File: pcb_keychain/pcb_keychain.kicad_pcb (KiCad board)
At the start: 11 copper layers, 84.3 x 60.5 mm, 7 parts, among them Q1 PN2222A, SW1 SW_SPDT

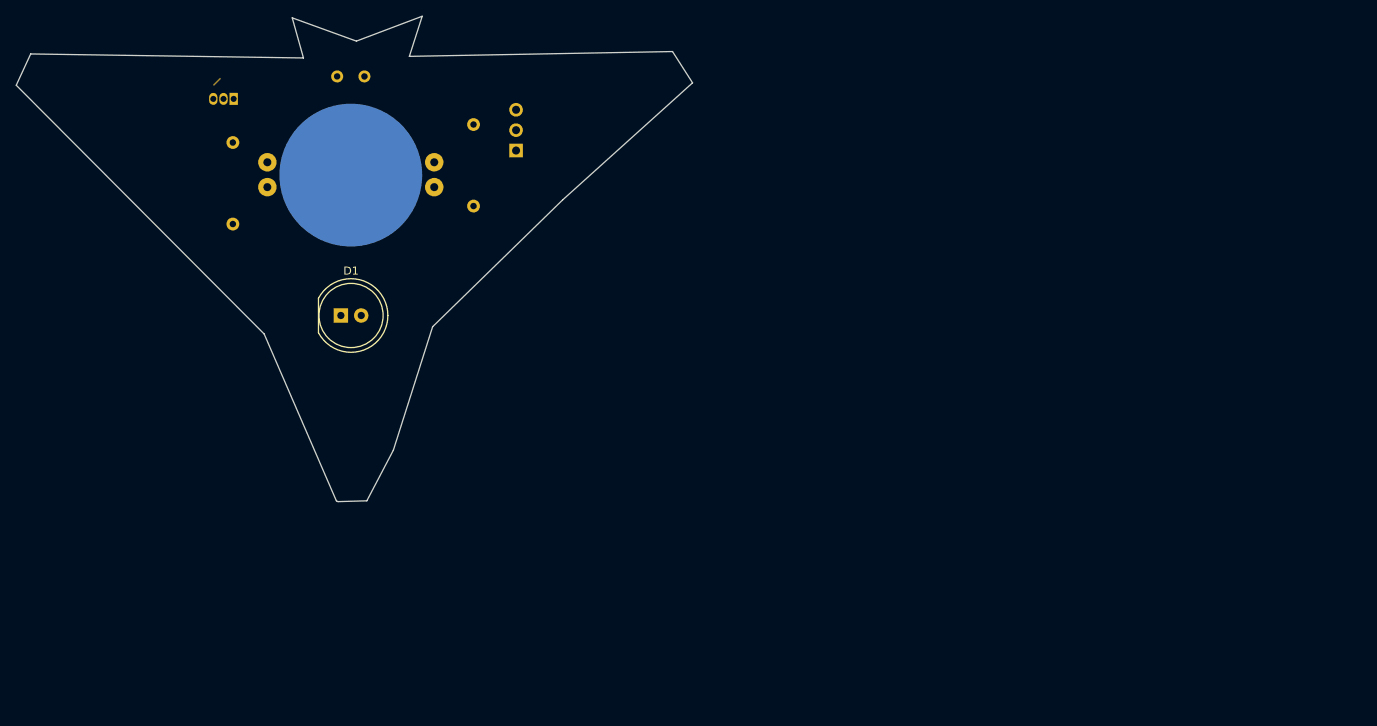
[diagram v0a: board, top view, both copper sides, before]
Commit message: v1 done. holy fk that was a sprint lmao
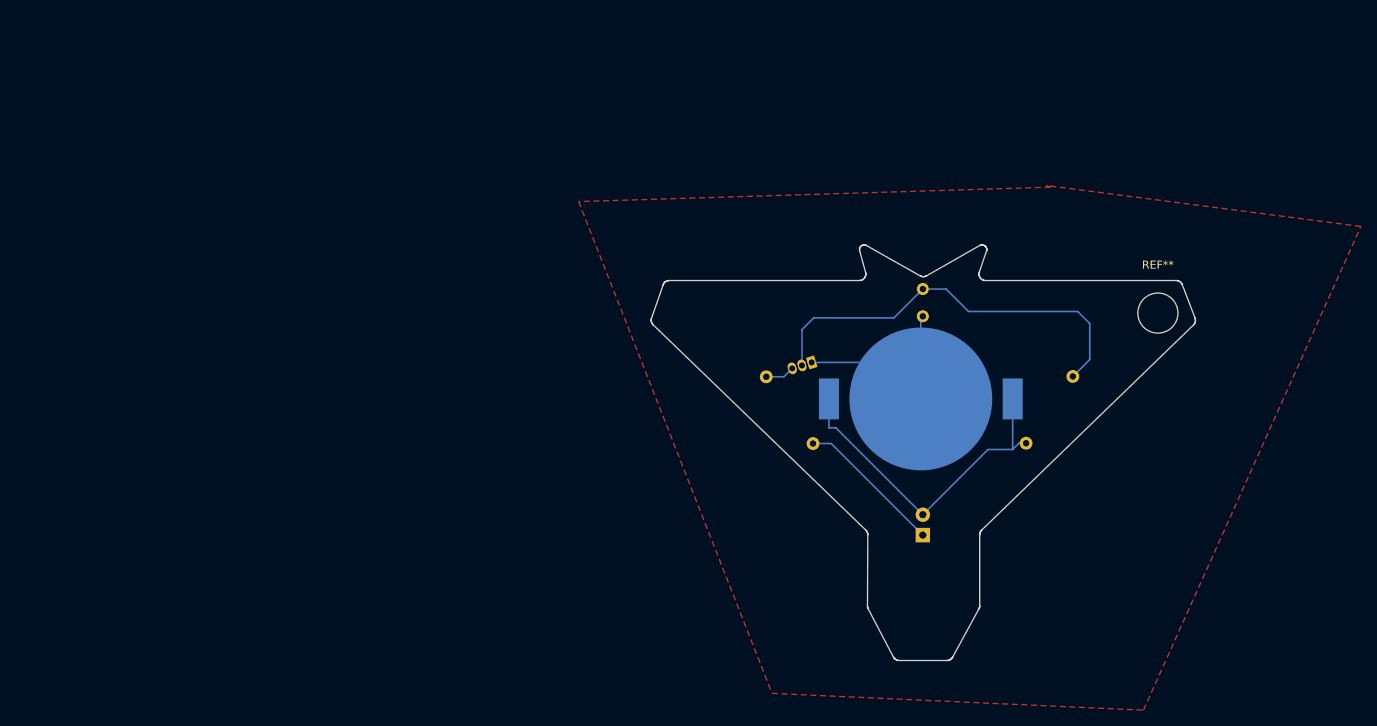
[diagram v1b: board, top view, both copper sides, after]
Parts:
- removed BT2: BAT-HLD-001-THM, BAT-HLD-001-THM:BAT_BAT-HLD-001-THM
- removed SW1: SW_SPDT, Connector_PinSocket_2.54mm:PinSocket_1x03_P2.54mm_Vertical
- added BT1: BAT-HLD-001, BAT-HLD-001:BAT_BAT-HLD-001, B.Cu at (226.2, 81.2)
- added REF**: MountingHole_5mm, MountingHole:MountingHole_5mm, F.Cu at (255.8, 70.5)
- moved R3 79.5 mm to (239.4, 86.7), turned to 55 degrees
- moved Q1 79.2 mm to (212.7, 76.7), turned to -163 degrees
- moved R2 77.7 mm to (226.5, 67.5), turned to -90 degrees
- moved D1 77.5 mm to (226.5, 98.2), turned to 90 degrees
- moved R1 77.3 mm to (212.8, 86.8), turned to 125 degrees
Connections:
- D1 pad 2: Net-(D1-A) -> VCC
- R3 pad 1: Net-(D1-A) -> VCC
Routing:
- net Net-(Q1-B): track 0.00 -> 51.7 mm
- net VCC: track 1.12 -> 42.8 mm
- net GND: track 0.00 -> 39.2 mm
- net Net-(D1-K): track 0.00 -> 18.4 mm
- net Net-(Q1-C): track 0.00 -> 3.67 mm
- added copper zone on F.Cu, net (none)
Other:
- board size 84.3 x 60.5 mm -> 67.8 x 51.8 mm
